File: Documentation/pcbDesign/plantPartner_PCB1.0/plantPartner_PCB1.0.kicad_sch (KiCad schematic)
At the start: 26 parts, among them IC1 MPM3610, J1 Conn_01x04, J2 Conn_01x04, J3 Conn_01x04, J4 Screw_Terminal, J5 Screw_Terminal, J6 Screw_Terminal, U1 ESP32-WROOM-32, U2 MAX485

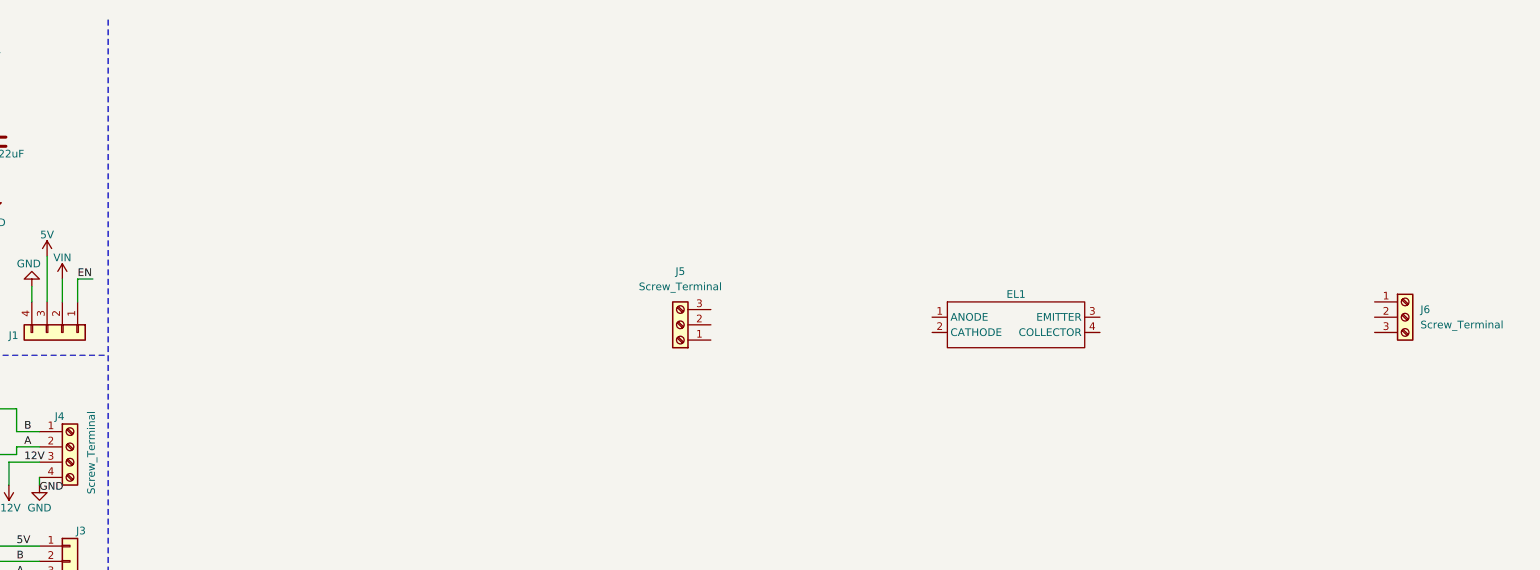
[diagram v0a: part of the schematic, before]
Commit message: Prototype demo changes. Small things for testing
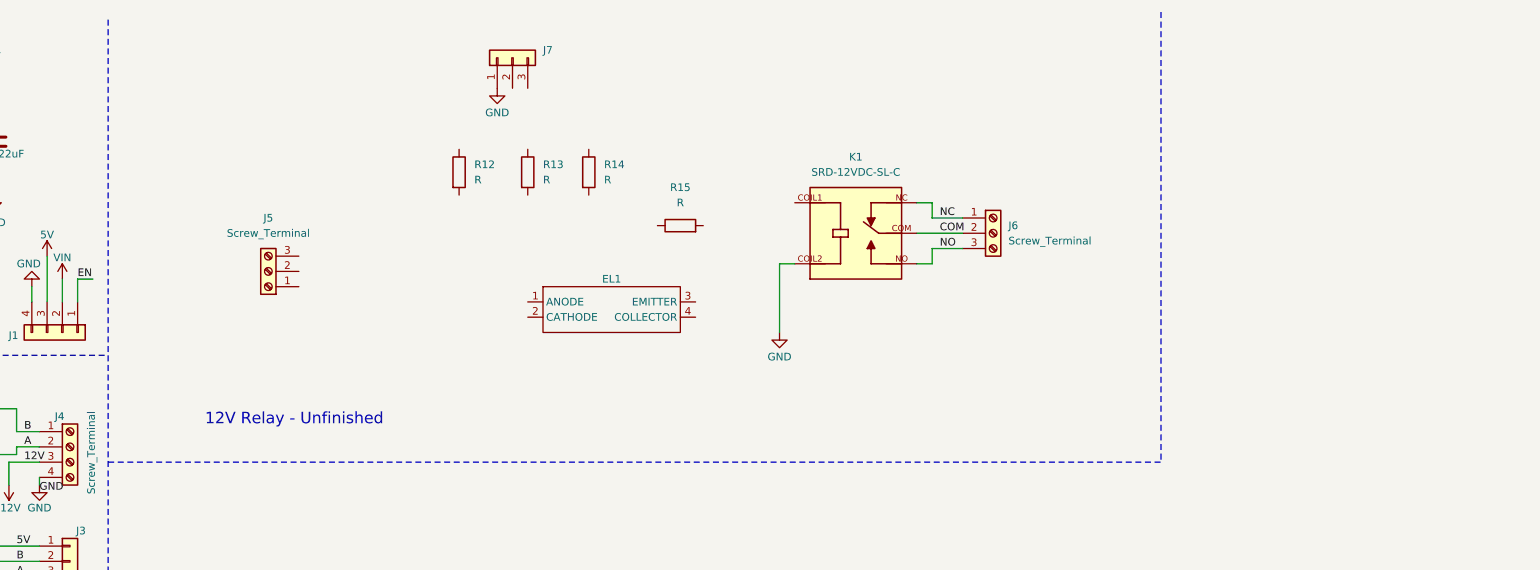
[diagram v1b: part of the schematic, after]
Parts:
- added J7: Conn_01x03, symbol Connector_Generic:Conn_01x03
- added K1: SRD-12VDC-SL-C, SRD-12VDC-SL-C:RELAY_SRD-12VDC-SL-C, symbol SRD-12VDC-SL-C:SRD-12VDC-SL-C
- added R12, R13, R14, R15: R, Resistor_SMD:R_0201_0603Metric, symbol Device:R
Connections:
- net GND: now also J7.1 (Pin_1), K1.COIL2
- net NC: now reaches J6.1 (Pin_1)
- net NC: now also K1.NC
- net COM: now reaches J6.2 (Pin_2)
- net COM: now also K1.COM
- net NO: now reaches J6.3 (Pin_3)
- net NO: now also K1.NO
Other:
- note added: "12V Relay - Unfinished"
- moved on the sheet: EL1, J5, J6
